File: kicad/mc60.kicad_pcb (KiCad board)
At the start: 2 copper layers, 60 x 70 mm, 107 parts, among them CN1 Conn_GPS, CN2 Conn_GNSS, CN3 SD_CARD, CN4 SIM_Card, CN5 Audio-Jack-4, CN6 5V_IN, J1 B_LS_N, J2 B_VRTC, J3 B_SPKP, J4 B_SPKN, J5 B_ADC, Q1 DTC114E, Q2 DTC114E, Q3 DTC114E, Q4 DTC143ZUA, U1 MC60_0, U2 TXB0108PWR, U3 MIC29302, U4 LP5907-3V3, U5 LP5907-2V8

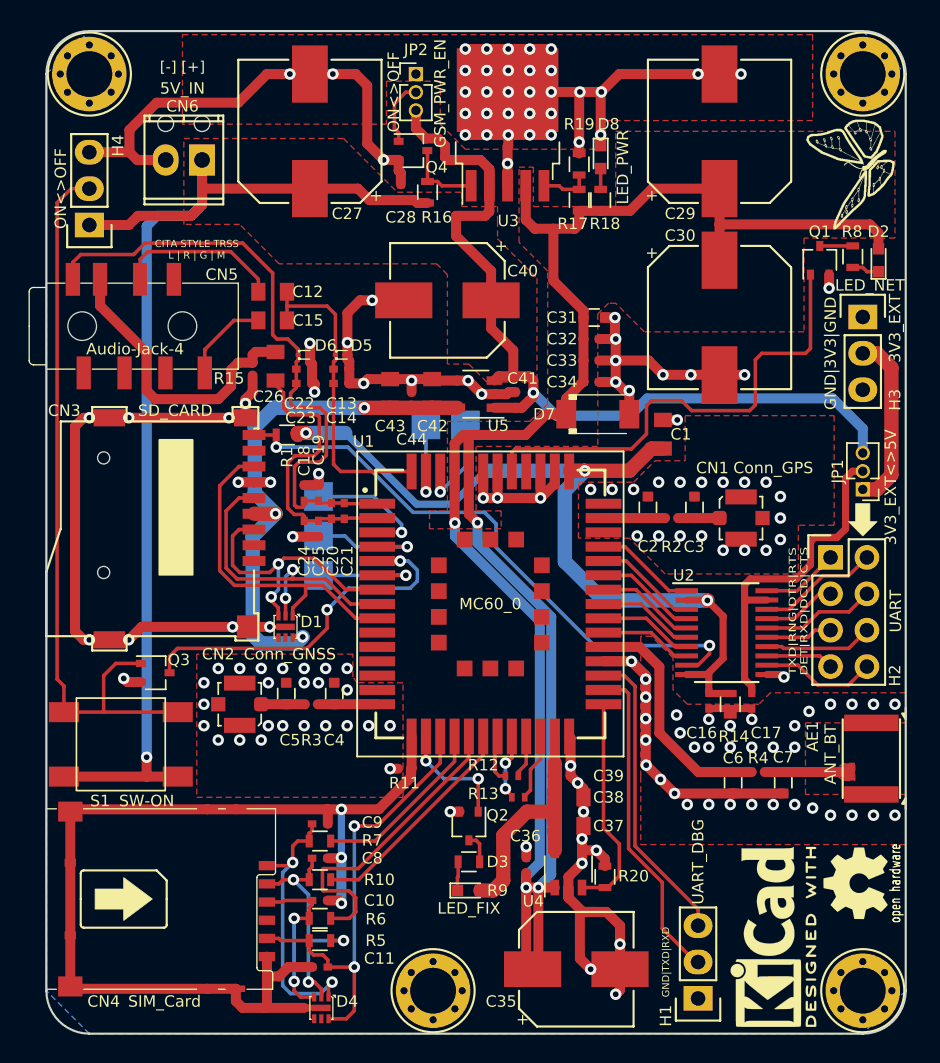
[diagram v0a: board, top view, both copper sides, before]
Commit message: layout wip
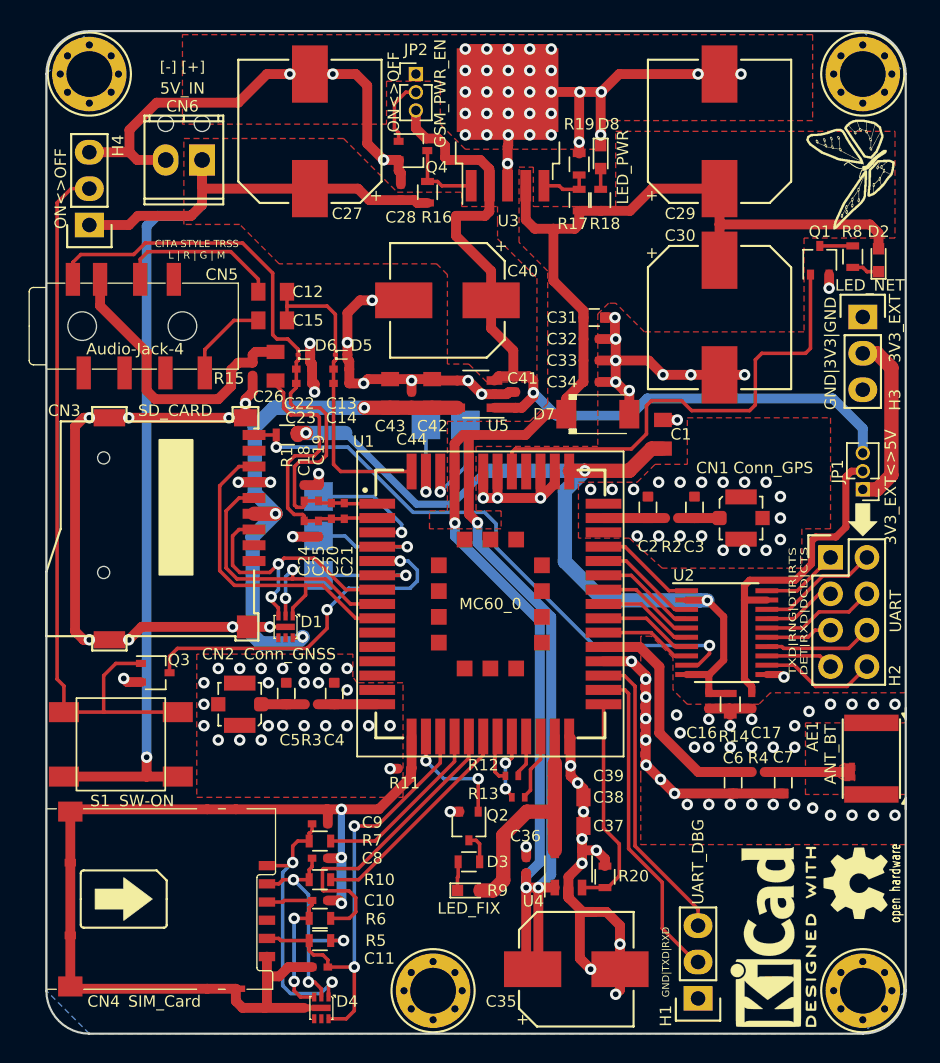
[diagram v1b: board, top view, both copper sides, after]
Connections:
- CN3 pad 1: Net-(CN3-Pad1) -> (no net)
- CN3 pad 2: Net-(CN3-Pad2) -> (no net)
- CN3 pad 8: Net-(CN3-Pad8) -> (no net)
- CN4 pad P6: Net-(CN4-PadP6) -> (no net)
- D1 pad 4: Net-(D1-Pad4) -> (no net)
- D1 pad 5: Net-(D1-Pad5) -> (no net)
- D4 pad 4: Net-(D4-Pad4) -> (no net)
- D4 pad 5: Net-(D4-Pad5) -> (no net)
- U1 pad 10: Net-(U1-Pad10) -> (no net)
- U1 pad 11: Net-(U1-Pad11) -> (no net)
- U1 pad 12: Net-(U1-Pad12) -> (no net)
- U1 pad 13: Net-(U1-Pad13) -> (no net)
- U1 pad 46: Net-(U1-Pad46) -> (no net)
- U1 pad 55: Net-(U1-Pad55) -> (no net)
- U1 pad 56: Net-(U1-Pad56) -> (no net)
- U1 pad 57: Net-(U1-Pad57) -> (no net)
- U1 pad 58: Net-(U1-Pad58) -> (no net)
- U1 pad 59: Net-(U1-Pad59) -> (no net)
- U1 pad 60: Net-(U1-Pad60) -> (no net)
- U1 pad 61: Net-(U1-Pad61) -> (no net)
- U1 pad 62: Net-(U1-Pad62) -> (no net)
- U1 pad 63: Net-(U1-Pad63) -> (no net)
- U1 pad 64: Net-(U1-Pad64) -> (no net)
- U1 pad 65: Net-(U1-Pad65) -> (no net)
- U1 pad 66: Net-(U1-Pad66) -> (no net)
- U1 pad 67: Net-(U1-Pad67) -> (no net)
- U1 pad 68: Net-(U1-Pad68) -> (no net)
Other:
- net class 0.70mm removed
- net class 0.72mm added: clearance 0.2, trace_width 0.69, via_dia 0.8, via_drill 0.4
- net class 0.7mmANT added: clearance 0.128, trace_width 0.7, via_dia 0.7, via_drill 0.4
- net class Default: clearance 0.2 -> 0.128
- rule trace_clearance: 0.2 -> 0.128
- rule trace_min: 0.2 -> 0.1
